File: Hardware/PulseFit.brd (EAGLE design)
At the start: 53.2 x 56.2 mm, 49 parts, among them SW1 SWITCH.JS202011JCQN

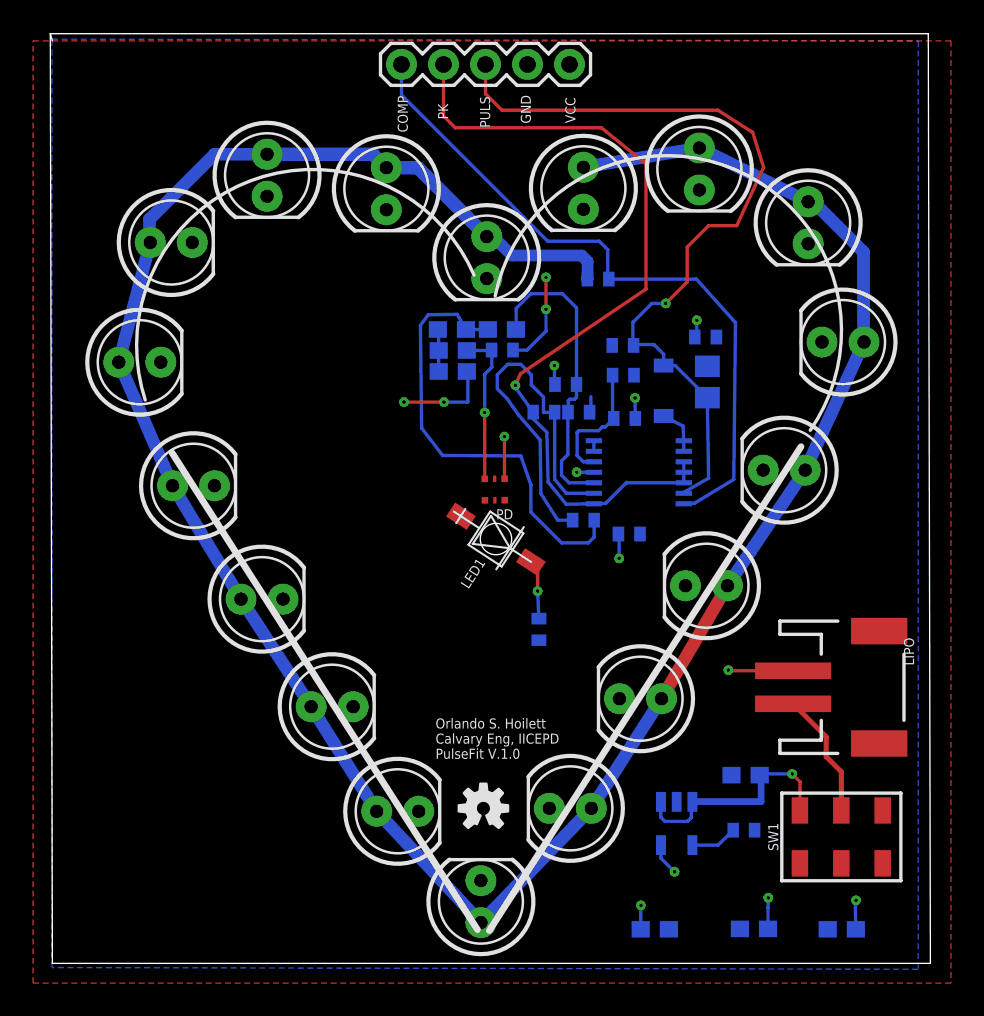
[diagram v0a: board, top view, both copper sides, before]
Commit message: next board
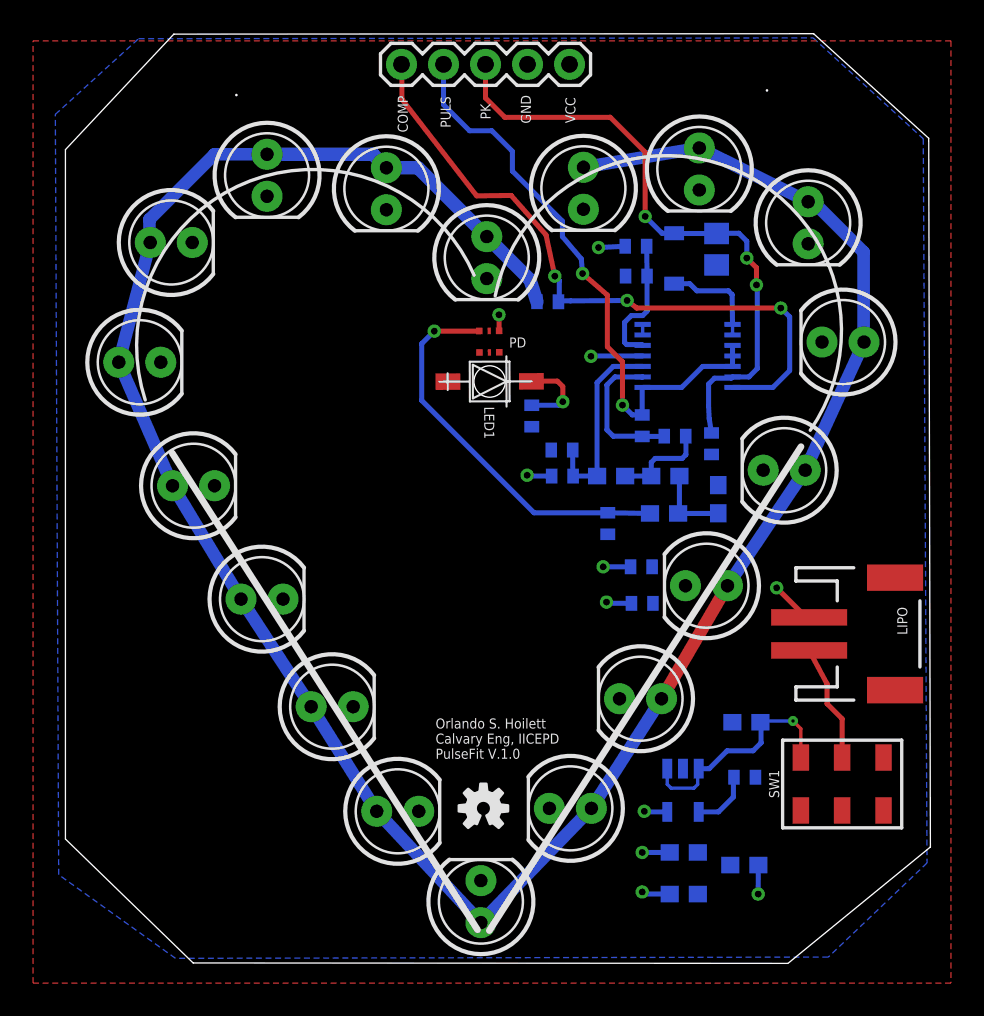
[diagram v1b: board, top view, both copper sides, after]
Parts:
- moved C8 17.8 mm to (64.8, 28.3), turned to 270 degrees
- moved C2 16.6 mm to (60.2, 22.0)
- moved C7 16.1 mm to (61.6, 27.5), turned to 180 degrees
- moved C9 15.7 mm to (61.6, 29.7), turned to 180 degrees
- moved R2 12.9 mm to (53.6, 33.4)
- moved R6 12.3 mm to (58.2, 26.8), turned to 90 degrees
- moved C6 11.1 mm to (58.4, 29.7), turned to 180 degrees
- moved R4 10.4 mm to (59.9, 43.6), turned to 0 degrees
- moved LED1 9.53 mm to (51.0, 35.4), turned to 0.2 degrees
- moved PD 8.95 mm to (51.0, 37.8)
- moved C10 8.05 mm to (64.7, 43.4), turned to 90 degrees
- moved D1 8.03 mm to (62.2, 42.9)
- moved R12 8.00 mm to (64.4, 31.7), turned to 270 degrees
- moved AMP 7.63 mm to (63.0, 37.0)
- moved R3 7.51 mm to (62.2, 32.1)
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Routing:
- net N$14: track 27.2 -> 5.81 mm
- net GND: track 18.9 -> 3.68 mm, vias 6 -> 2
- net PULSE: track 51.1 -> 36.2 mm, vias 1 -> 2
- net N$15: track 23.6 -> 8.75 mm
- net N$18: track 9.55 -> 23.9 mm
- net PEAK: track 49.3 -> 38.0 mm, vias 1 -> 3
- net N$17: track 18.4 -> 11.8 mm
- net N$10: track 2.84 -> 6.22 mm
- net 3.3V: track 13.1 -> 16.0 mm
- net ANODE: track 148.3 -> 145.5 mm
- net N$13: track 2.56 -> 4.72 mm
- net N$9: track 3.61 -> 4.92 mm
- net COMP: track 41.7 -> 40.4 mm, vias 0 -> 3
- net N$3: track 2.84 -> 3.68 mm
- net N$4: track 7.66 -> 7.13 mm
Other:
- board size 53.2 x 56.2 mm -> 52.3 x 56.2 mm
